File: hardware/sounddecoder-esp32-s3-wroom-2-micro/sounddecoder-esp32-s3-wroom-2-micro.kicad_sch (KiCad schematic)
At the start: 36 parts, among them J1 Input power, J10 AUX1, J11 AUX2, J12 AUX3, J13 AUX4, J2 Boot, J3 Motor, J4 Speaker, J5 UART, J6 Conn_01x03_Pin, J7 Smoke, J8 FwdLED, J9 BackLED, U1 LM2596S-5, U3 MAX98357A, U4 DRV8871DDA, U5 W25Q256, U6 AMS1117-3.3, U7 ESP32-S3-WROOM-1, U8 ULN2003A

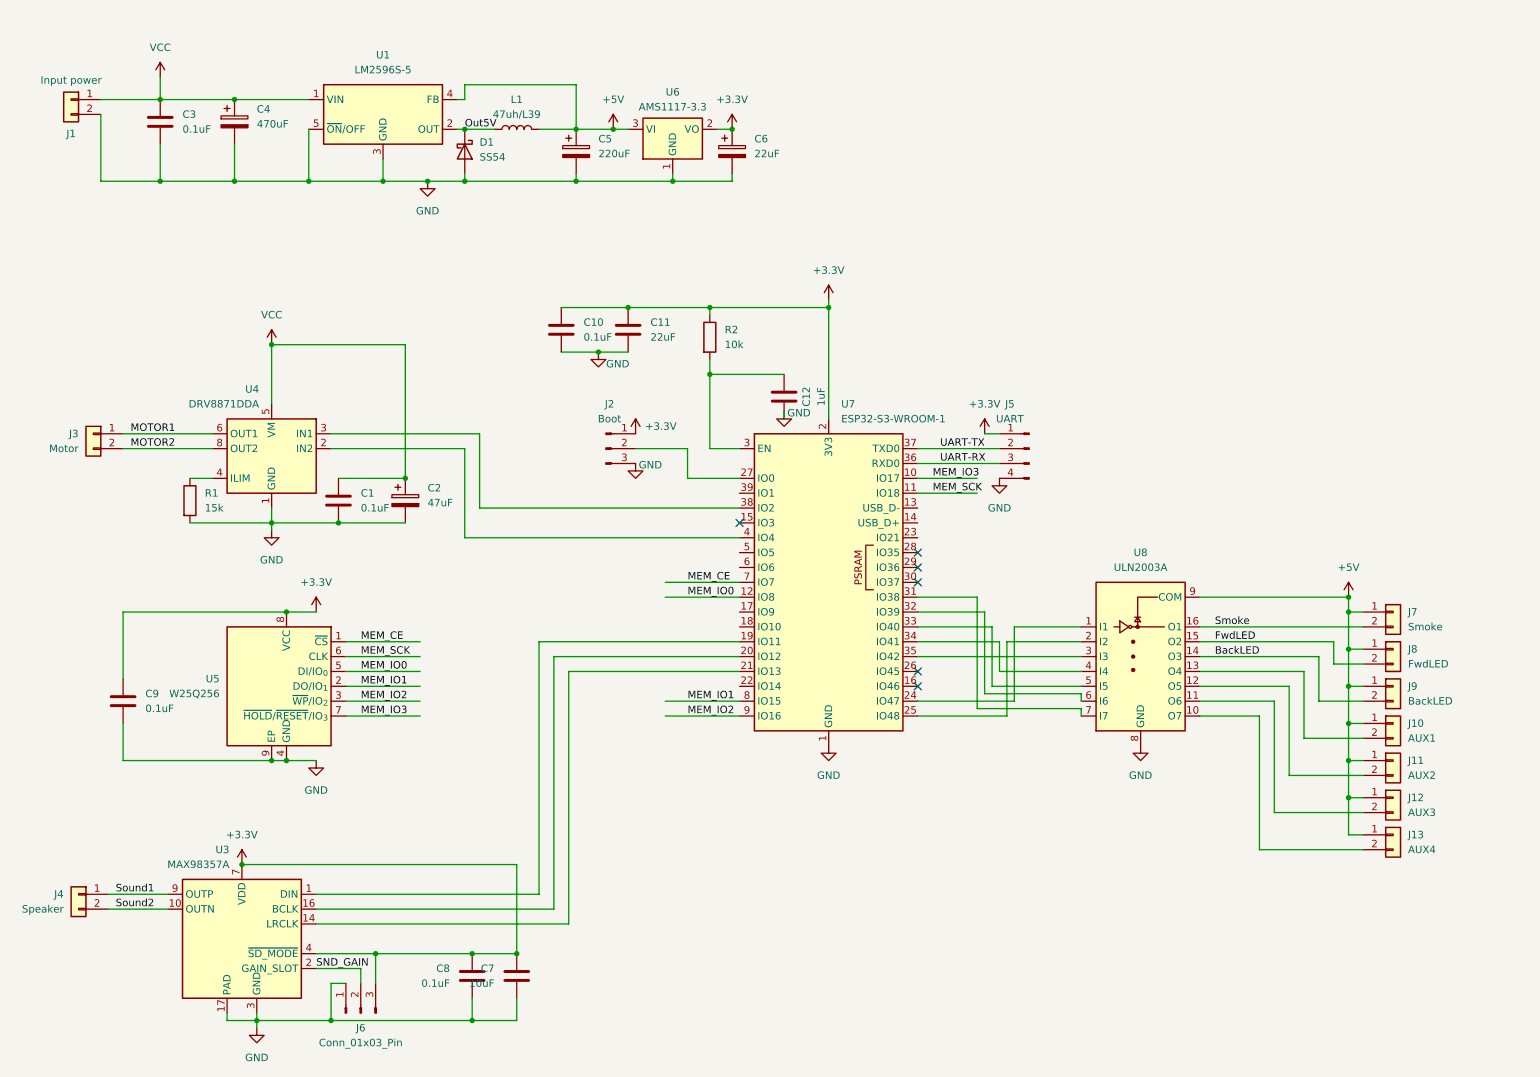
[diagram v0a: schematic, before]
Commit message: Added micro board
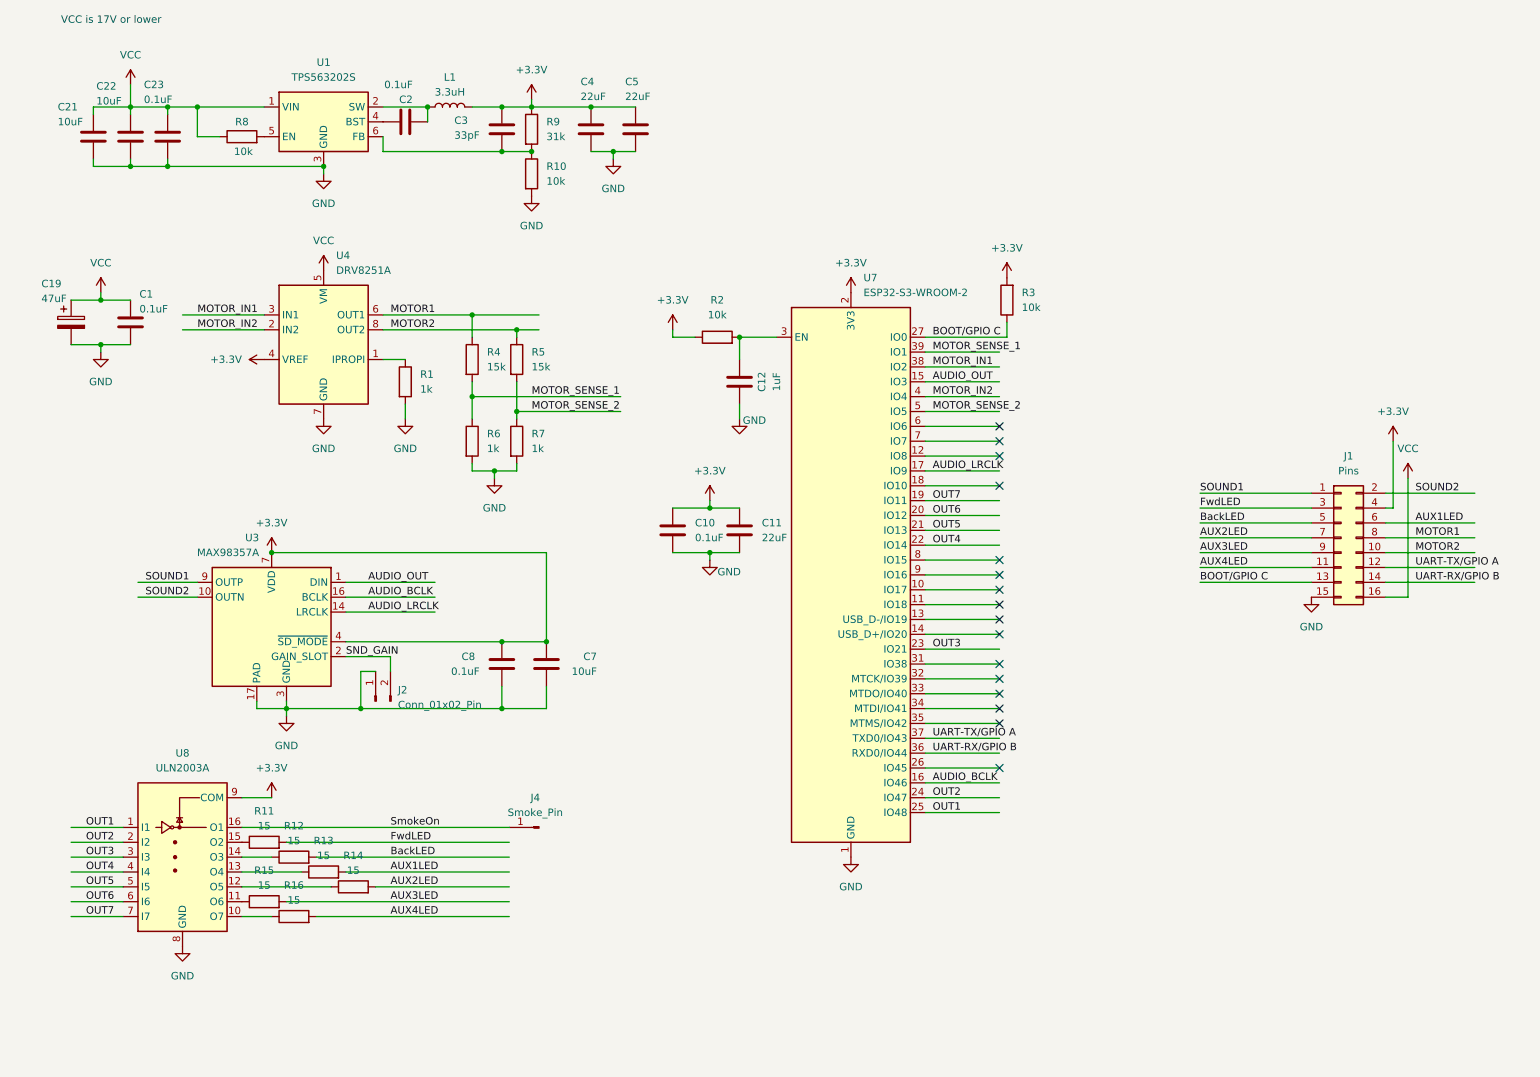
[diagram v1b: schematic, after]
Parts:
- removed C2: 47uF, Capacitor_SMD:CP_Elec_6.3x5.4, symbol Device:C_Polarized
- removed C4: 470uF, Capacitor_SMD:CP_Elec_10x10.5, symbol Device:C_Polarized
- removed C5: 220uF, Capacitor_SMD:C_Elec_6.3x7.7, symbol Device:C_Polarized
- removed C6: 22uF, Capacitor_SMD:CP_Elec_4x5.4, symbol Device:C_Polarized
- removed C9: 0.1uF, Capacitor_SMD:C_0805_2012Metric_Pad1.18x1.45mm_HandSolder, symbol Device:C
- removed D1: SS54, Diode_SMD:D_SMC, symbol Diode:1N5822
- removed J1: Input power, TerminalBlock:TerminalBlock_Xinya_XY308-2.54-2P_1x02_P2.54mm_Horizontal, symbol Connector_Generic:Conn_01x02
- removed J10: AUX1, TerminalBlock:TerminalBlock_Xinya_XY308-2.54-2P_1x02_P2.54mm_Horizontal, symbol Connector_Generic:Conn_01x02
- removed J11: AUX2, TerminalBlock:TerminalBlock_Xinya_XY308-2.54-2P_1x02_P2.54mm_Horizontal, symbol Connector_Generic:Conn_01x02
- removed J12: AUX3, TerminalBlock:TerminalBlock_Xinya_XY308-2.54-2P_1x02_P2.54mm_Horizontal, symbol Connector_Generic:Conn_01x02
- removed J13: AUX4, TerminalBlock:TerminalBlock_Xinya_XY308-2.54-2P_1x02_P2.54mm_Horizontal, symbol Connector_Generic:Conn_01x02
- removed J2: Boot, Connector_PinHeader_1.00mm:PinHeader_1x03_P1.00mm_Vertical, symbol Connector:Conn_01x03_Pin
- removed J3: Motor, TerminalBlock:TerminalBlock_Xinya_XY308-2.54-2P_1x02_P2.54mm_Horizontal, symbol Connector_Generic:Conn_01x02
- removed J4: Speaker, TerminalBlock:TerminalBlock_Xinya_XY308-2.54-2P_1x02_P2.54mm_Horizontal, symbol Connector_Generic:Conn_01x02
- removed J5: UART, Connector_PinSocket_2.54mm:PinSocket_1x04_P2.54mm_Horizontal, symbol Connector:Conn_01x04_Pin
- removed J6: Conn_01x03_Pin, Connector_PinHeader_1.00mm:PinHeader_1x03_P1.00mm_Vertical, symbol Connector:Conn_01x03_Pin
- removed J7: Smoke, TerminalBlock:TerminalBlock_Xinya_XY308-2.54-2P_1x02_P2.54mm_Horizontal, symbol Connector_Generic:Conn_01x02
- removed J8: FwdLED, TerminalBlock:TerminalBlock_Xinya_XY308-2.54-2P_1x02_P2.54mm_Horizontal, symbol Connector_Generic:Conn_01x02
- removed J9: BackLED, TerminalBlock:TerminalBlock_Xinya_XY308-2.54-2P_1x02_P2.54mm_Horizontal, symbol Connector_Generic:Conn_01x02
- removed U1: LM2596S-5, Package_TO_SOT_SMD:TO-263-5_TabPin3, symbol Regulator_Switching:LM2596S-5
- removed U4: DRV8871DDA, Package_SO:Texas_HTSOP-8-1EP_3.9x4.9mm_P1.27mm_EP2.95x4.9mm_Mask2.4x3.1mm_ThermalVias, symbol Driver_Motor:DRV8871DDA
- removed U5: W25Q256, Package_SON:WSON-8-1EP_8x6mm_P1.27mm_EP3.4x4.3mm, symbol Memory_Flash:W25Q128JVP
- removed U6: AMS1117-3.3, Package_TO_SOT_SMD:SOT-223-3_TabPin2, symbol Regulator_Linear:AMS1117-3.3
- removed U7: ESP32-S3-WROOM-1, RF_Module:ESP32-S3-WROOM-1, symbol RF_Module:ESP32-S3-WROOM-1
- added C19: 47uF, Capacitor_SMD:CP_Elec_6.3x5.4, symbol Device:C_Polarized
- added C2, C23: 0.1uF, Capacitor_SMD:C_0603_1608Metric, symbol Device:C
- added C21, C22: 10uF, Capacitor_SMD:C_0603_1608Metric, symbol Device:C
- added C4, C5: 22uF, Capacitor_SMD:C_0603_1608Metric, symbol Device:C
- added J1: Pins, Connector_PinHeader_2.00mm:PinHeader_2x08_P2.00mm_Vertical, symbol Connector_Generic:Conn_02x08_Odd_Even
- added J2: Conn_01x02_Pin, Jumper:SolderJumper-2_P1.3mm_Open_RoundedPad1.0x1.5mm, symbol Connector:Conn_01x02_Pin
- added J4: Smoke_Pin, TestPoint:TestPoint_THTPad_1.0x1.0mm_Drill0.5mm, symbol Connector:Conn_01x01_Pin
- added R10, R3, R8: 10k, Capacitor_SMD:C_0603_1608Metric, symbol Device:R
- added R11, R12, R13, R14, R15, R16: 15, Capacitor_SMD:C_0603_1608Metric, symbol Device:R
- added R4, R5: 15k, Capacitor_SMD:C_0603_1608Metric, symbol Device:R
- added R6, R7: 1k, Capacitor_SMD:C_0603_1608Metric, symbol Device:R
- added R9: 31k, Capacitor_SMD:C_0603_1608Metric, symbol Device:R
- added U1: TPS563202S, Package_TO_SOT_SMD:SOT-563, symbol Regulator_Switching:TPS563202S
- added U4: DRV8251A, Package_SO:Texas_HSOP-8-1EP_3.9x4.9mm_P1.27mm_ThermalVias, symbol Driver_Motor:DRV8231ADSG
- added U7: ESP32-S3-WROOM-2, RF_Module:ESP32-S3-WROOM-2, symbol RF_Module:ESP32-S3-WROOM-2
- C1, C10, C11, C12, C7, C8: footprint Capacitor_SMD:C_0805_2012Metric_Pad1.18x1.45mm_HandSolder -> Capacitor_SMD:C_0603_1608Metric
- C3: value 0.1uF -> 33pF; footprint Capacitor_SMD:C_0805_2012Metric_Pad1.18x1.45mm_HandSolder -> Capacitor_SMD:C_0603_1608Metric
- L1: value 47uh/L39 -> 3.3uH; footprint Inductor_SMD:L_Bourns_SRP1245A -> Inductor_SMD:L_Chilisin_BMRA00050530
- R1: value 15k -> 1k; footprint Resistor_SMD:R_0805_2012Metric_Pad1.20x1.40mm_HandSolder -> Capacitor_SMD:C_0603_1608Metric
- R2: footprint Resistor_SMD:R_0805_2012Metric_Pad1.20x1.40mm_HandSolder -> Capacitor_SMD:C_0603_1608Metric
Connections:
- net +5V is gone; now on net +3.3V: L1.2, U8.9 (COM)
- net +3.3V: now also C3.1, C4.1, C5.1, J1.4 (Pin_4), R3.2, R9.1, U4.4 (VREF), U7.2 (3V3)
- net BackLED: now also J1.5 (Pin_5), R12.2; no longer U8.14 (O3)
- net FwdLED: now also J1.3 (Pin_3), R11.2; no longer U8.15 (O2)
- net GND: now also C19.2, C21.2, C22.2, C23.2, C4.2, C5.2, J1.15 (Pin_15), J2.1 (Pin_1), R10.2, R6.2, R7.2, U1.3 (GND), U4.7 (GND), U4.9 (GND), U7.1 (GND), U7.40 (GND), U7.41 (GND); no longer C3.2
- net MOTOR1: now also J1.8 (Pin_8), R4.1, U4.6 (OUT1)
- net MOTOR2: now also J1.10 (Pin_10), R5.1, U4.8 (OUT2)
- net SND_GAIN: now also J2.2 (Pin_2)
- net VCC: now also C19.1, C21.1, C22.1, C23.1, J1.16 (Pin_16), R8.1, U1.1 (VIN), U4.5 (VM); no longer C3.1
- net AUDIO_OUT: now reaches U3.1 (DIN)
- net AUDIO_OUT: now also U7.15 (IO3)
- net AUDIO_LRCLK: now reaches U3.14 (LRCLK)
- net AUDIO_LRCLK: now also U7.17 (IO9)
- net AUDIO_BCLK: now reaches U3.16 (BCLK)
- net AUDIO_BCLK: now also U7.16 (IO46)
- net at R1.1: now also U4.1 (IPROPI)
- net OUT1: now reaches U8.1 (I1)
- net OUT1: now also U7.25 (IO48)
- net at U8.10 (O7): now also R16.1
- net at U8.11 (O6): now also R15.1
- net at U8.12 (O5): now also R14.1
- net at U8.13 (O4): now also R13.1
- net OUT2: now reaches U8.2 (I2)
- net OUT2: now also U7.24 (IO47)
- net OUT3: now reaches U8.3 (I3)
- net OUT3: now also U7.23 (IO21)
- net OUT4: now reaches U8.4 (I4)
- net OUT4: now also U7.22 (IO14)
- net OUT5: now reaches U8.5 (I5)
- net OUT5: now also U7.21 (IO13)
- net OUT6: now reaches U8.6 (I6)
- net OUT6: now also U7.20 (IO12)
- net OUT7: now reaches U8.7 (I7)
- net OUT7: now also U7.19 (IO11)
- net at C12.2, R2.2: now also U7.3 (EN)
- net Out5V: no longer names the net of L1.1
- net Out5V: now also C2.2, U1.2 (SW)
- net Smoke renamed SmokeOn
- net SmokeOn: now also J4.1 (Pin_1)
- net Sound1 renamed SOUND1
- net SOUND1: now also J1.1 (Pin_1)
- net Sound2 renamed SOUND2
- net SOUND2: now also J1.2 (Pin_2)
- new net: R12.1, U8.14 (O3)
- new net: R11.1, U8.15 (O2)
- new net: C2.1, U1.4 (BST)
- new net: R8.2, U1.5 (EN)
- new net: C3.2, R10.1, R9.2, U1.6 (FB)
- new net AUX1LED: J1.6 (Pin_6), R13.2
- new net AUX2LED: J1.7 (Pin_7), R14.2
- new net AUX3LED: J1.9 (Pin_9), R15.2
- new net AUX4LED: J1.11 (Pin_11), R16.2
- new net BOOT/GPIO C: J1.13 (Pin_13), R3.1, U7.27 (IO0)
- new net MOTOR_IN1: U4.3 (IN1), U7.38 (IO2)
- new net MOTOR_IN2: U4.2 (IN2), U7.4 (IO4)
- new net MOTOR_SENSE_1: R4.2, R6.1, U7.39 (IO1)
- new net MOTOR_SENSE_2: R5.2, R7.1, U7.5 (IO5)
- new net UART-RX/GPIO B: J1.14 (Pin_14), U7.36 (RXD0/IO44)
- new net UART-TX/GPIO A: J1.12 (Pin_12), U7.37 (TXD0/IO43)
- no-connect marks 6 -> 16
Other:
- note added: "VCC is 17V or lower"
- moved on the sheet: C1, C10, C11, C12, C7, C8, R1, R2, U3, U8
